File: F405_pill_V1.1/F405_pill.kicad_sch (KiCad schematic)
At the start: 53 parts, among them J1 Conn_01x04_Male, J2 Conn_01x04_Male, J4 TYPE-C-31-M-12, J5 Conn_01x02, U1 STM32F405VGTx, U2 TJA1050T/CM,118, U3 LM1117-3.3, U4 STM32F405_pill, U5 HT7550, Y1 8MHz

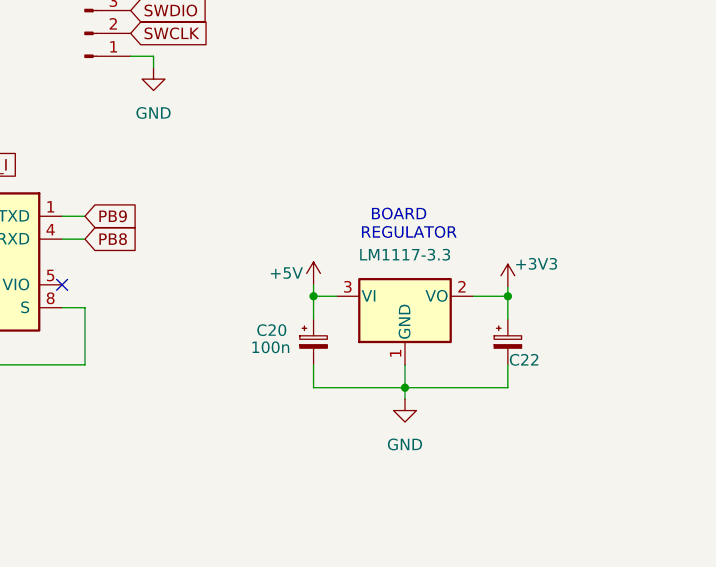
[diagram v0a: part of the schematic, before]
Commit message: updated for prodaction
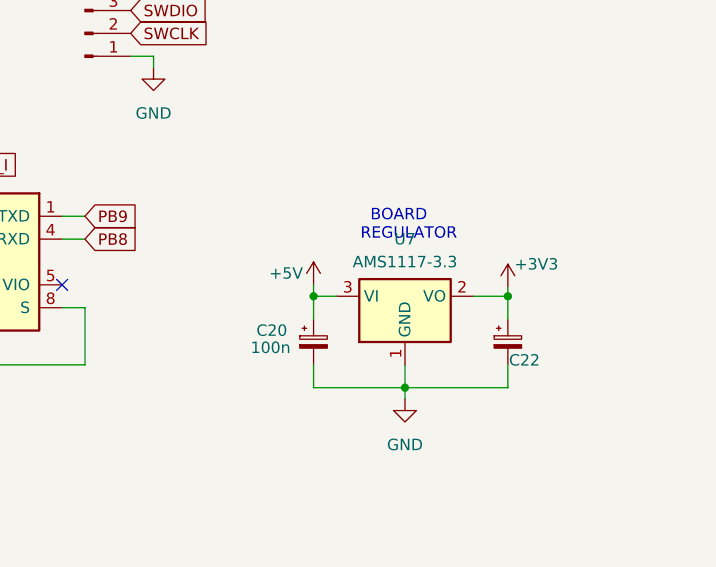
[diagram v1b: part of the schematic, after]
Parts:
- removed U3: LM1117-3.3, Package_TO_SOT_SMD:SOT-223-3_TabPin2, symbol Regulator_Linear:LM1117-3.3
- added U7: AMS1117-3.3, Package_TO_SOT_SMD:SOT-223-3_TabPin2, symbol Regulator_Linear:AMS1117-3.3
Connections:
- net +3V3: now also U7.2 (VO)
- net +5V: now also U7.3 (VI)
- net GND: now also U7.1 (GND)
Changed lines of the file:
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@@
-	)
-	(symbol
-		(lib_id "Regulator_Linear:LM1117-3.3")
-		(at 378.46 224.79 0)
-		(unit 1)
-		(exclude_from_sim no)
-		(in_bom yes)
-		(on_board yes)
-		(dnp no)
-		(fields_autoplaced yes)
-		(property "Reference" "U3"
-			(at 378.46 217.17 0)
-			(effects
-				(font
-					(size 1.27 1.27)
-				)
-				(hide yes)
-			)
-		)
-		(property "Value" "LM1117-3.3"
-			(at 378.46 220.218 0)
-			(effects
-				(font
-					(size 1.27 1.27)
-				)
-			)
-		)
-		(property "Footprint" "Package_TO_SOT_SMD:SOT-223-3_TabPin2"
-			(at 378.46 224.79 0)
-			(effects
-				(font
-					(size 1.27 1.27)
-				)
-				(hide yes)
-			)
-		)
-		(property "Datasheet" "https://datasheet.lcsc.com/lcsc/1811131822_HTC-Korea-TAEJIN-Tech-LM1117S-3-3_C126027.pdf"
-			(at 378.46 224.79 0)
-			(effects
-				(font
-					(size 1.27 1.27)
-				)
-				(hide yes)
-			)
-		)
-		(property "Description" ""
-			(at 378.46 224.79 0)
-			(effects
-				(font
-					(size 1.27 1.27)
-				)
-				(hide yes)
-			)
-		)
-		(property "LCSC" "C126027"
-			(at 378.46 224.79 0)
-			(effects
-				(font
-					(size 1.27 1.27)
-				)
-				(hide yes)
-			)
-		)
-		(pin "1"
-		)
-		(pin "2"
-		)
-		(pin "3"
-		)
-		(instances
-			(project "F405_pill"
-				(path "/e63e39d7-6ac0-4ffd-8aa3-1841a4541b55"
-					(reference "U3")
-					(unit 1)
-				)
-			)
-		)
 	)
 	(symbol
@@
 					(unit 1)
 				)
+			)
+		)
+	)
+	(symbol
+		(lib_id "Regulator_Linear:AMS1117-3.3")
+		(at 378.46 224.79 0)
+		(unit 1)
+		(exclude_from_sim no)
+		(in_bom yes)
+		(on_board yes)
+		(dnp no)
+		(fields_autoplaced yes)
+		(property "Reference" "U7"
+			(at 378.46 218.44 0)
+			(effects
+				(font
+					(size 1.27 1.27)
+				)
+			)
+		)
+		(property "Value" "AMS1117-3.3"
+			(at 378.46 220.98 0)
+			(effects
+				(font
+					(size 1.27 1.27)
+				)
+			)
+		)
+		(property "Footprint" "Package_TO_SOT_SMD:SOT-223-3_TabPin2"
+			(at 378.46 219.71 0)
+			(effects
+				(font
+					(size 1.27 1.27)
+				)
+				(hide yes)
+			)
+		)
+		(property "Datasheet" "http://www.advanced-monolithic.com/pdf/ds1117.pdf"
+			(at 381 231.14 0)
+			(effects
+				(font
+					(size 1.27 1.27)
+				)
+				(hide yes)
+			)
+		)
+		(property "Description" "1A Low Dropout regulator, positive, 3.3V fixed output, SOT-223"
+			(at 378.46 224.79 0)
+			(effects
+				(font
+					(size 1.27 1.27)
+				)
+				(hide yes)
+			)
+		)
+		(property "MPN" "C6186"
+			(at 378.46 224.79 0)
+			(effects
+				(font
+					(size 1.27 1.27)
+				)
+				(hide yes)
+			)
+		)
+		(pin "3"
+		)
+		(pin "2"
+		)
+		(pin "1"
+		)
+		(instances
+			(project ""
+				(path "/e63e39d7-6ac0-4ffd-8aa3-1841a4541b55"
+					(reference "U7")
+					(unit 1)
+				)
